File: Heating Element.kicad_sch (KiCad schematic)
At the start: 21 parts, among them IC1 UCC23513QDWYRQ1, J1 Conn_01x02_Pin, J2 Conn_01x02_Pin, U1 STP55NF06L, U2 MC7815CDTRKG

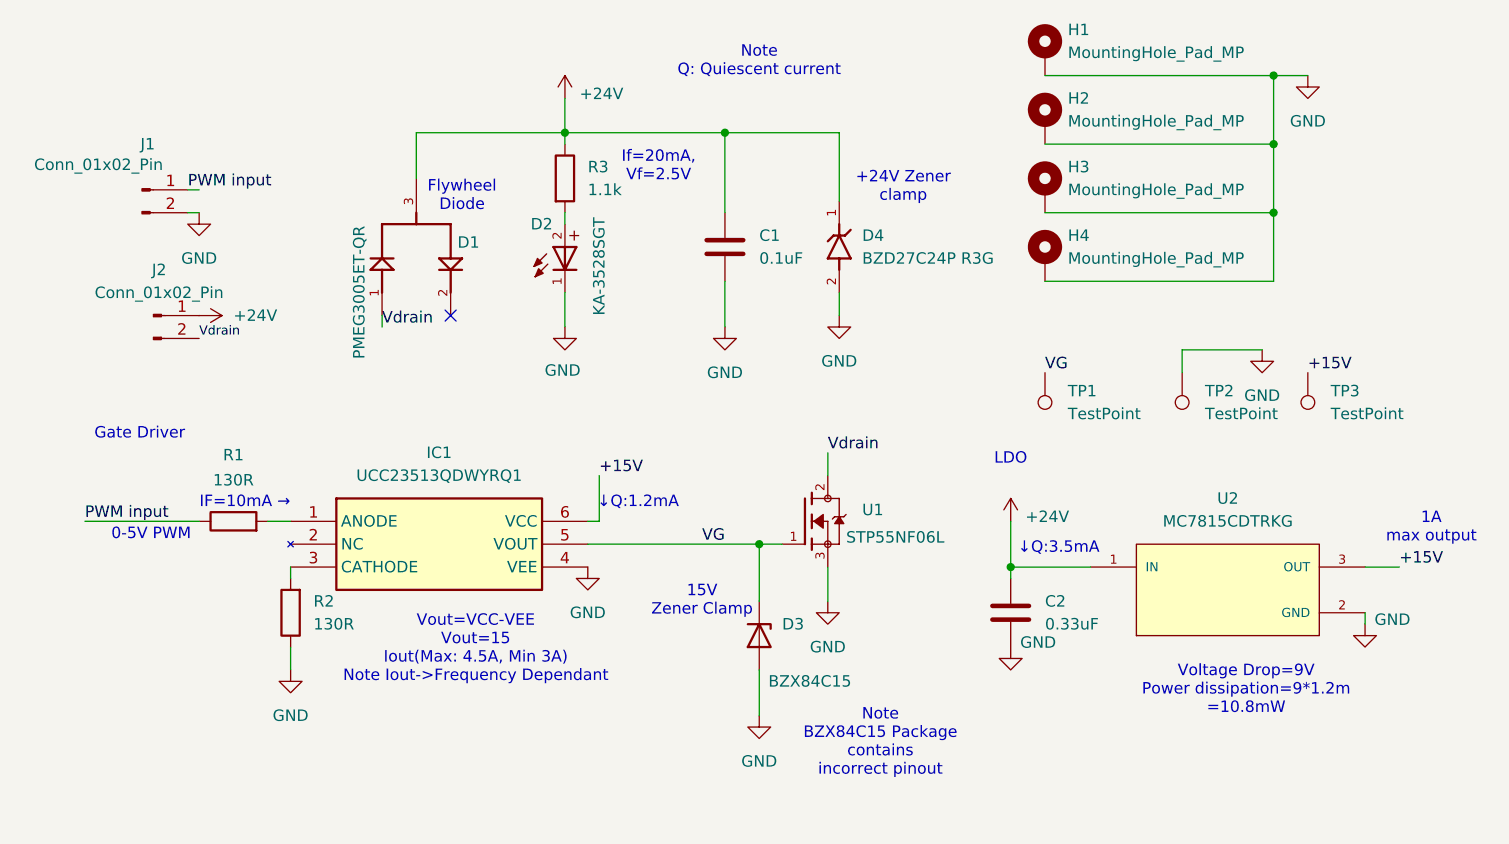
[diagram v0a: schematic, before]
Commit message: updated Heating PCB
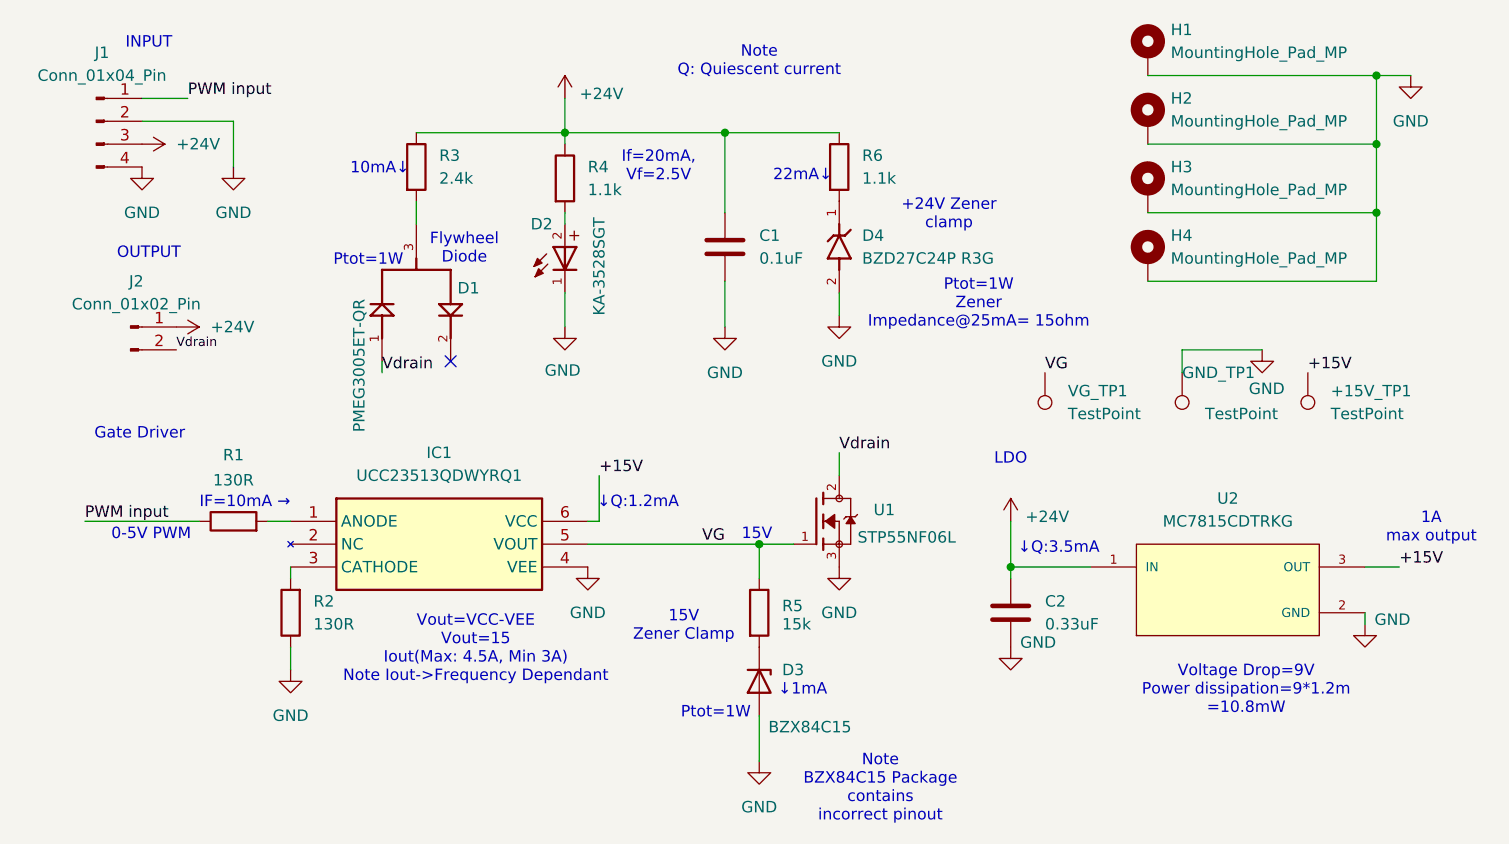
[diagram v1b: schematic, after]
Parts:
- removed J1: Conn_01x02_Pin, Connector_PinSocket_2.00mm:PinSocket_1x02_P2.00mm_Vertical, symbol Connector:Conn_01x02_Pin
- added J1: Conn_01x04_Pin, Connector_PinSocket_2.54mm:PinSocket_1x04_P2.54mm_Vertical, symbol Connector:Conn_01x04_Pin
- added R3: 2.4k, Resistor_SMD:R_1206_3216Metric, symbol Device:R
- added R5: 15k, Resistor_SMD:R_1206_3216Metric, symbol Device:R
- added R6: 1.1k, Resistor_SMD:R_1206_3216Metric, symbol Device:R
- J2: footprint Connector_PinSocket_2.00mm:PinSocket_1x02_P2.00mm_Vertical -> Connector_PinHeader_2.54mm:PinHeader_1x02_P2.54mm_Vertical
- renumbered TP3 to +15V_TP1, TP2 to GND_TP1, R3 to R4, TP1 to VG_TP1
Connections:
- net +24V: now also J1.3 (Pin_3), R3.1, R6.1; no longer D1.3, D4.1
- net GND: now also J1.2 (Pin_2), J1.4 (Pin_4)
- net PWM input: now also J1.1 (Pin_1)
- net VG: now also R5.1; no longer D3.3 (K)
- new net: D4.1, R6.2
- new net: D1.3, R3.2
- new net: D3.3 (K), R5.2
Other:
- note added: "10mA↓"
- note added: "15V"
- note added: "22mA↓"
- note added: "INPUT"
- note added: "OUTPUT"
- note added: "Ptot=1W"
- note added: "Ptot=1W Zener Impedance@25mA= 15ohm"
- note added: "↓1mA"
- moved on the sheet: D1, D3, H1, H2, H3, H4, J2, U1
